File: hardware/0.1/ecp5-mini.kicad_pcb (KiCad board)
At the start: 4 copper layers, 52 x 27 mm, 102 parts, among them J1 Micro_SD_Card, J2 JTAG, J3 S7 Mini, J4 S7 Mini, J5 USB_C_Receptacle_USB2.0, Q1 BSS138, Q2 BSS138, Q3 BSS138, Q4 BSS138, SW1 SW_Push, U1 ECP5U_12_CABGA256, U2 TLV73325PDBV, U3 TLV62568DBV, U4 USBLC6-2SC6, U5 TLV62568DBV, U6 W25Q128JVSIQ, U7 S27KL0641, X1 DSC6101CI2A-016

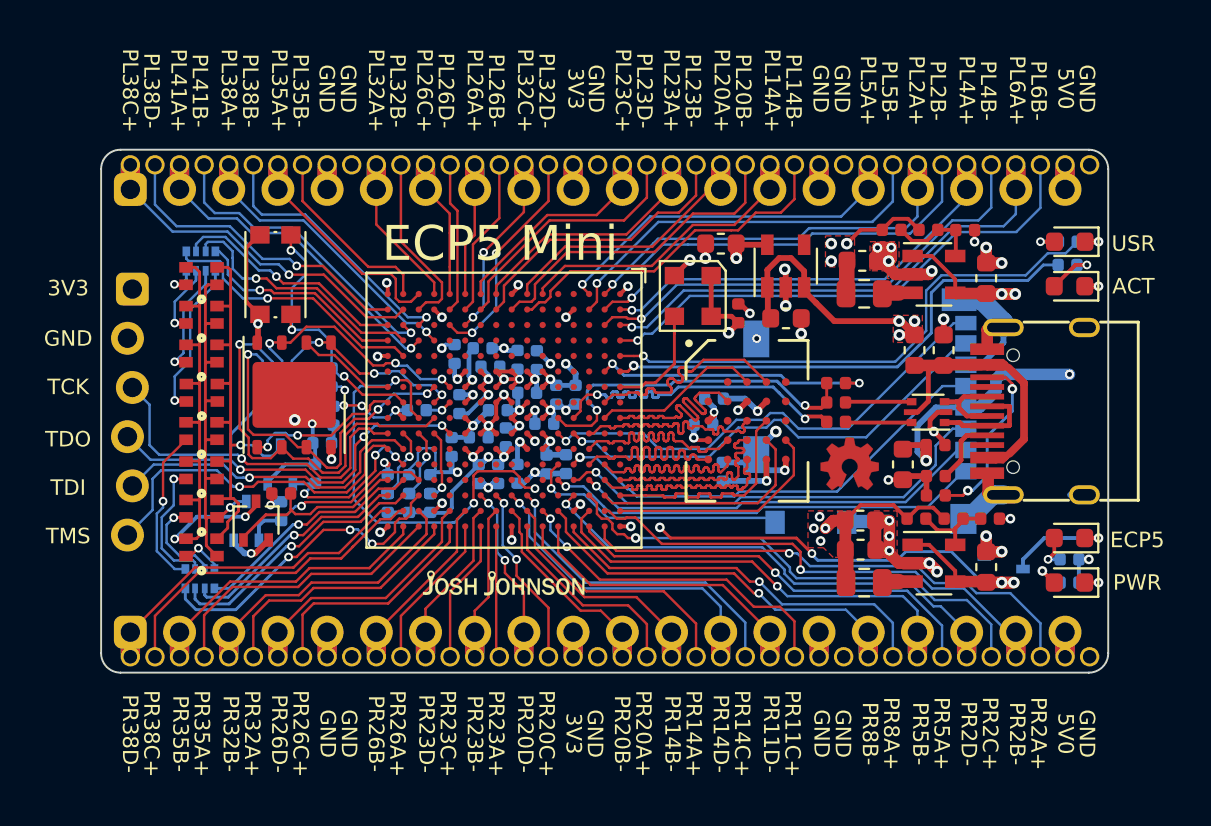
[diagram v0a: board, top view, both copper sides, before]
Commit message: update readme
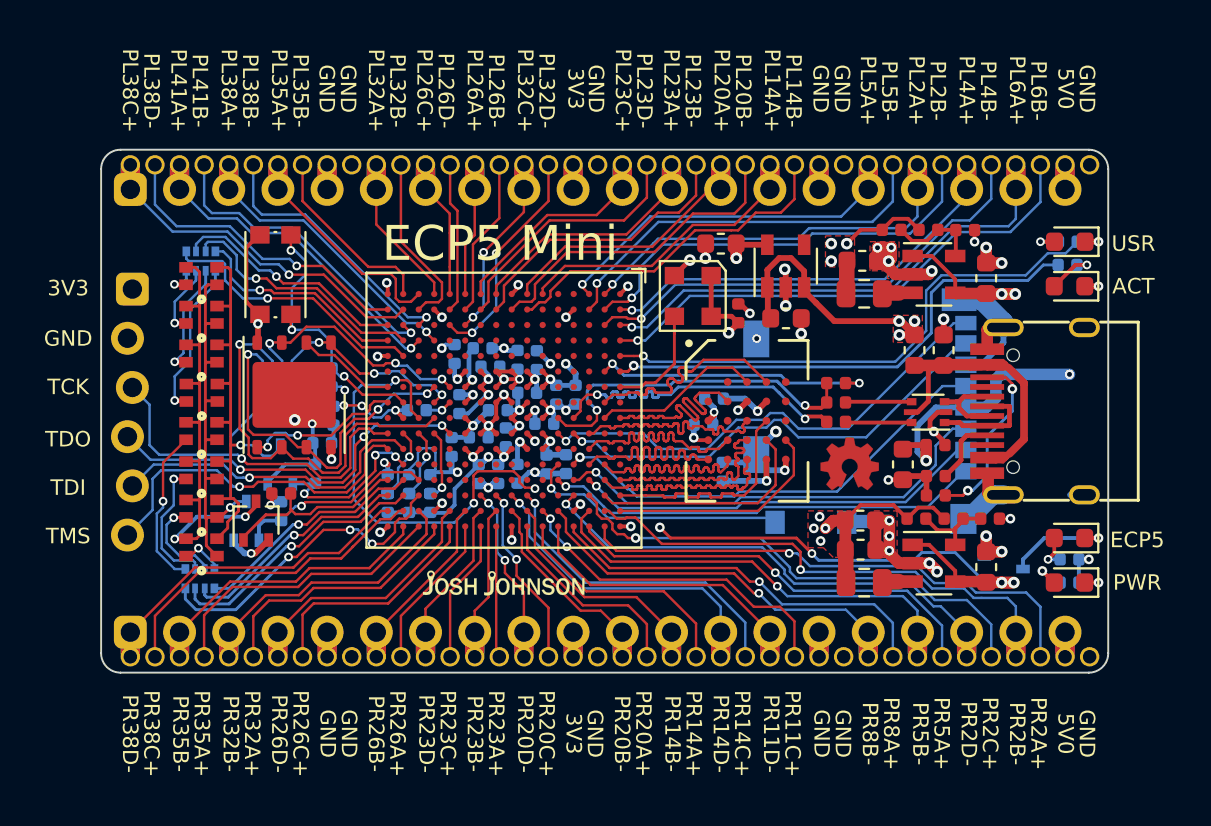
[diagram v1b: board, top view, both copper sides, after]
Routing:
- net /PORT_D3: track 24.4 -> 25.2 mm
